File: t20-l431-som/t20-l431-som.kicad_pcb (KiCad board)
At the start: 4 copper layers, 10.1 x 12.2 mm, 54 parts, among them U1 STM32L431-WLCSP64, U2 T20W80, U3 MX25U3232F, U4 MODULE_INTERNAL_T20_L431_HOST, U5 LP3986TL-2518/NOPB, U6 74LVC1T45_DSBGA_YZP, U7 TPS22916BYFPR, U8 SIT8021AI-J4-XXS-16.000000, U9 NCP139AFCT120T2G

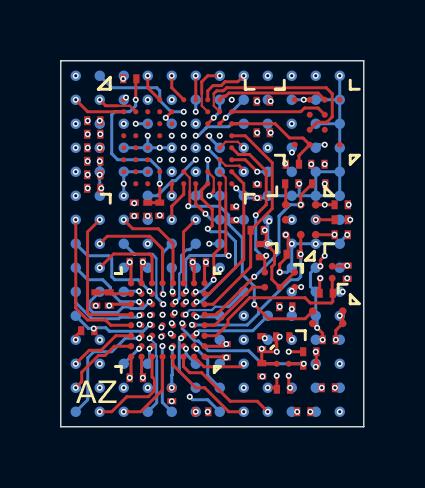
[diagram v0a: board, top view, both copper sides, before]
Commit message: Final design ready to order
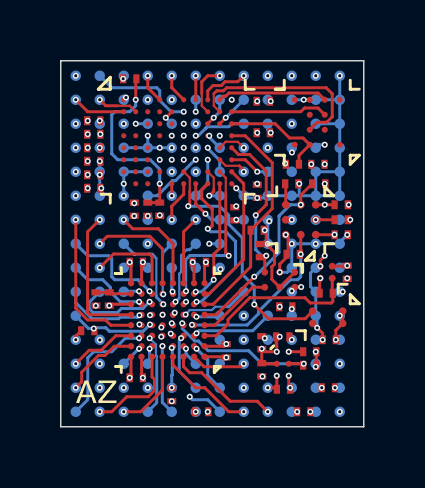
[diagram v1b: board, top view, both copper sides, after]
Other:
- rule pad_to_mask_clearance: 0 -> 0.05
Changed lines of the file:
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@@
 			(dielectric_constraints no)
 		)
-		(pad_to_mask_clearance 0)
+		(pad_to_mask_clearance 0.05)
 		(allow_soldermask_bridges_in_footprints no)
 		(tenting front back)
@@
 	)
 	(segment
-		(start 83.67543 75.191423)
-		(end 84.493627 75.191423)
-		(width 0.1)
-		(layer "B.Cu")
-		(net 96)
-	)
-	(segment
-		(start 84.949999 75.059025)
-		(end 85.336235 75.059025)
-		(width 0.1)
-		(layer "B.Cu")
-		(net 96)
-	)
-	(segment
-		(start 84.493627 75.191423)
-		(end 84.676024 75.009026)
+		(start 83.543629 75.059622)
+		(end 83.543629 74.856371)
 		(width 0.1)
 		(layer "B.Cu")
@@
 	)
 	(segment
-		(start 83.543629 74.856371)
-		(end 83.543629 75.059622)
+		(start 85.336235 75.059025)
+		(end 84.626025 75.059025)
 		(width 0.1)
 		(layer "B.Cu")
@@
 	)
 	(segment
-		(start 84.9 75.009026)
-		(end 84.949999 75.059025)
+		(start 85.561233 74.834025)
+		(end 85.336235 75.059025)
 		(width 0.1)
 		(layer "B.Cu")
@@
 	)
 	(segment
-		(start 83.543629 75.059622)
+		(start 84.493627 75.191423)
 		(end 83.67543 75.191423)
 		(width 0.1)
@@
 	)
 	(segment
-		(start 85.336235 75.059025)
-		(end 85.561233 74.834025)
+		(start 84.626025 75.059025)
+		(end 84.493627 75.191423)
 		(width 0.1)
 		(layer "B.Cu")
@@
 	)
 	(segment
-		(start 84.676024 75.009026)
-		(end 84.9 75.009026)
+		(start 83.543629 74.856371)
+		(end 83.9 74.5)
 		(width 0.1)
 		(layer "B.Cu")
@@
 	)
 	(segment
-		(start 83.9 74.5)
-		(end 83.543629 74.856371)
+		(start 83.67543 75.191423)
+		(end 83.543629 75.059622)
 		(width 0.1)
 		(layer "B.Cu")
